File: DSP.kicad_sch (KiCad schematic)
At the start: 24 parts, among them J10 USB to Serial, J11 LCD, Q4 2N3904-SMD, Q5 2N3904-SMD, Q6 AO3400A, SW1 RST, SW2 Frequency, SW3 Menu, SW4 BOOT, U6 ESP32-A1S

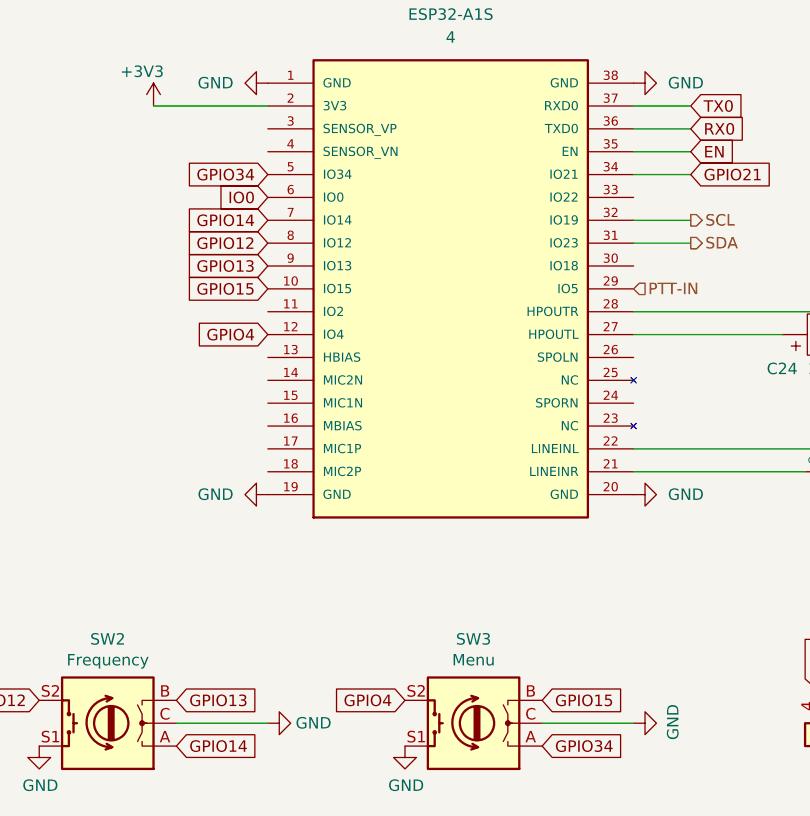
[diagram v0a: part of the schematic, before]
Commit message: moved GPIO34 to GPIO2 for encoder
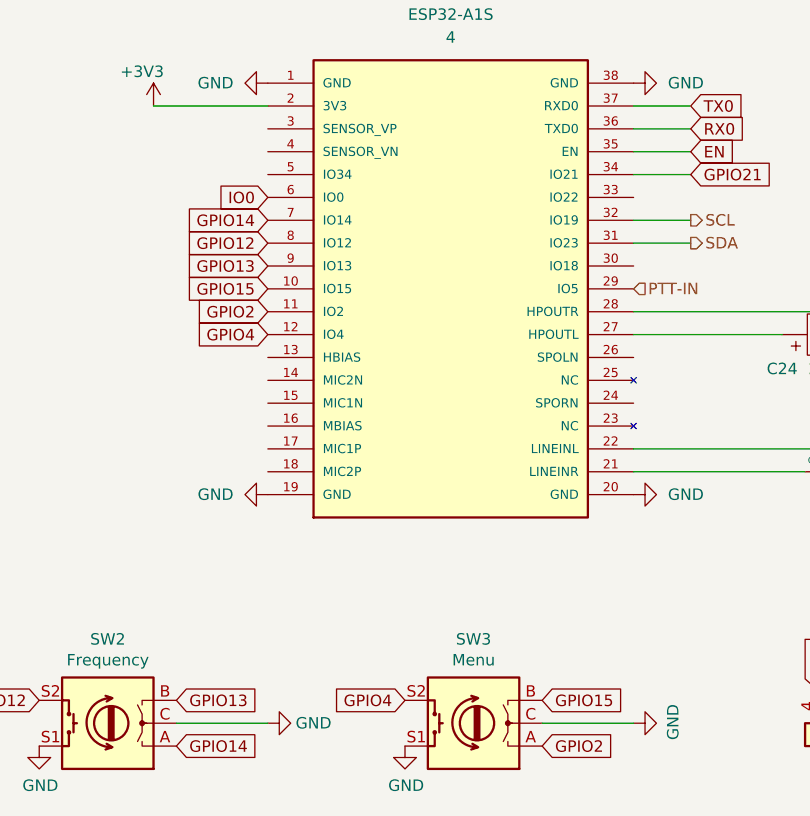
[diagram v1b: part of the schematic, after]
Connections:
- net GPIO2: now reaches U6.11 (IO2)
- net GPIO2: now also SW3.A
- net GPIO34: no longer names the net of U6.5 (IO34)
- net GPIO34: no longer SW3.A
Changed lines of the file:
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@@
     )
   )
-  (global_label "GPIO34" (shape input) (at 118.11 85.09 180) (fields_autoplaced)
+  (global_label "GPIO2" (shape input) (at 118.11 100.33 180) (fields_autoplaced)
     (effects (font (size 1.27 1.27)) (justify right))
-    (property "Intersheet References" "${INTERSHEET_REFS}" (id 0) (at 108.8026 85.1694 0)
+    (property "Intersheet References" "${INTERSHEET_REFS}" (id 0) (at 110.0121 100.2506 0)
       (effects (font (size 1.27 1.27)) (justify right) hide)
     )
@@
     )
   )
+  (global_label "GPIO2" (shape input) (at 148.59 148.59 0) (fields_autoplaced)
+    (effects (font (size 1.27 1.27)) (justify left))
+    (property "Intersheet References" "${INTERSHEET_REFS}" (id 0) (at 156.6879 148.6694 0)
+      (effects (font (size 1.27 1.27)) (justify left) hide)
+    )
+  )
   (global_label "GPIO14" (shape input) (at 118.11 90.17 180) (fields_autoplaced)
     (effects (font (size 1.27 1.27)) (justify right))
@@
       (effects (font (size 1.27 1.27)) (justify left) hide)
     )
-  )
-  (global_label "GPIO34" (shape input) (at 148.59 148.59 0) (fields_autoplaced)
-    (effects (font (size 1.27 1.27)) (justify left))
-    (property "Intersheet References" "${INTERSHEET_REFS}" (id 0) (at 157.8974 148.5106 0)
-      (effects (font (size 1.27 1.27)) (justify left) hide)
-    )
